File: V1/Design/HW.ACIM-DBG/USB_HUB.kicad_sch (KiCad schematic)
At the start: 45 parts, among them J1 USB C, U1 LDO 3.3V, U2 USB HUB 2.0 4-CH, Y1 24MHz

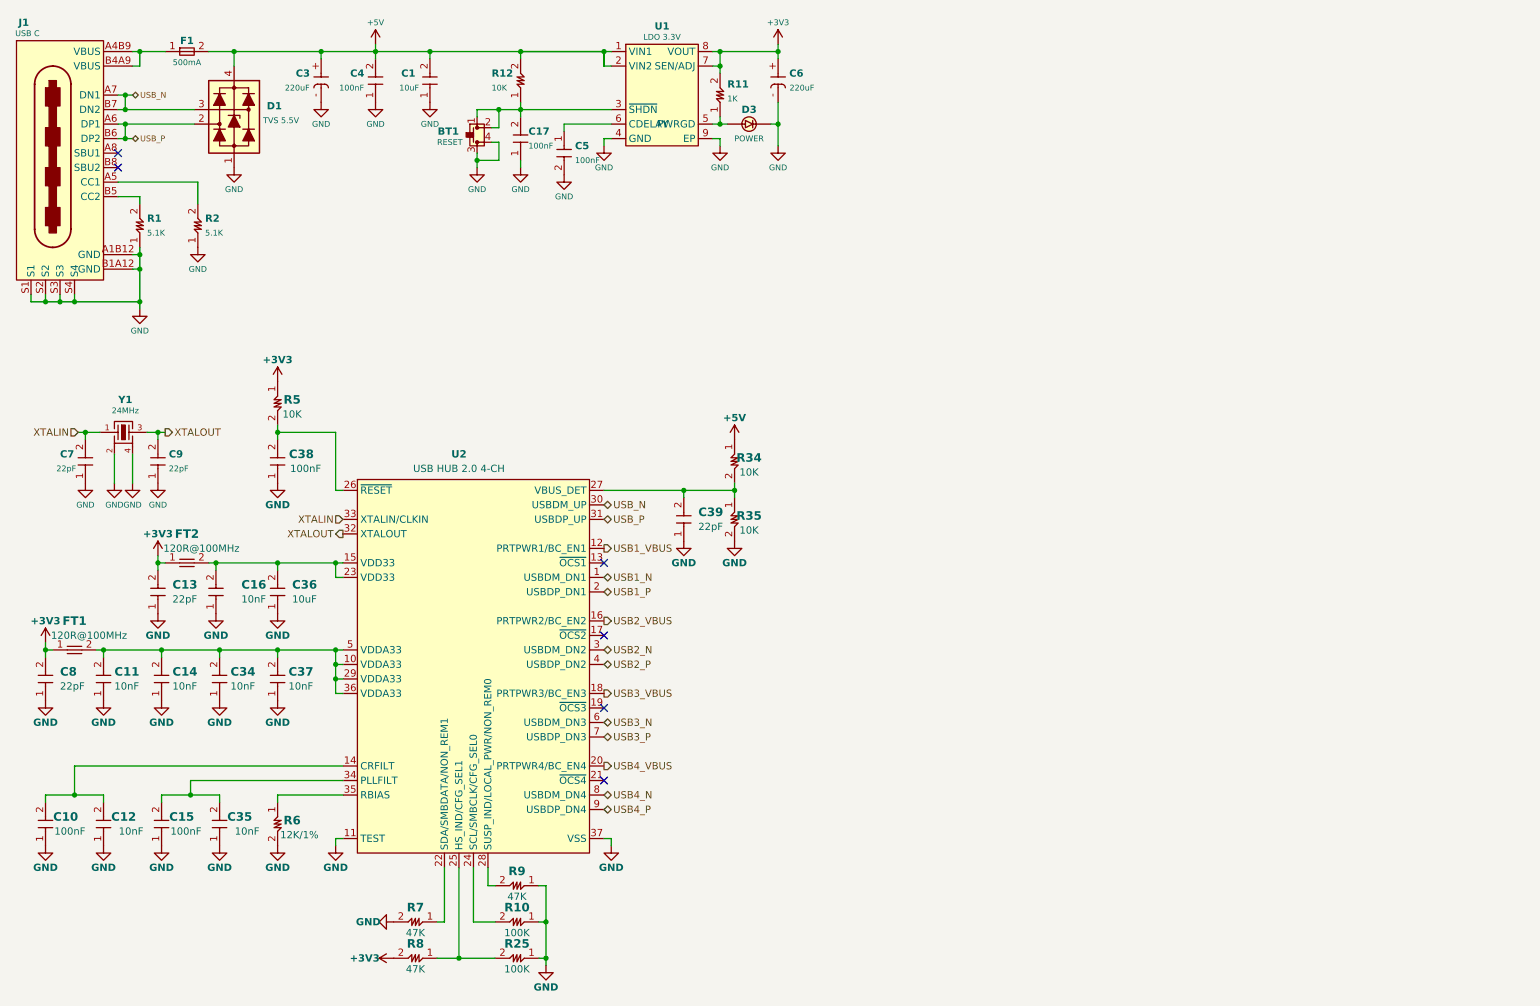
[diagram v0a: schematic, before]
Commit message: V1 layout update 6
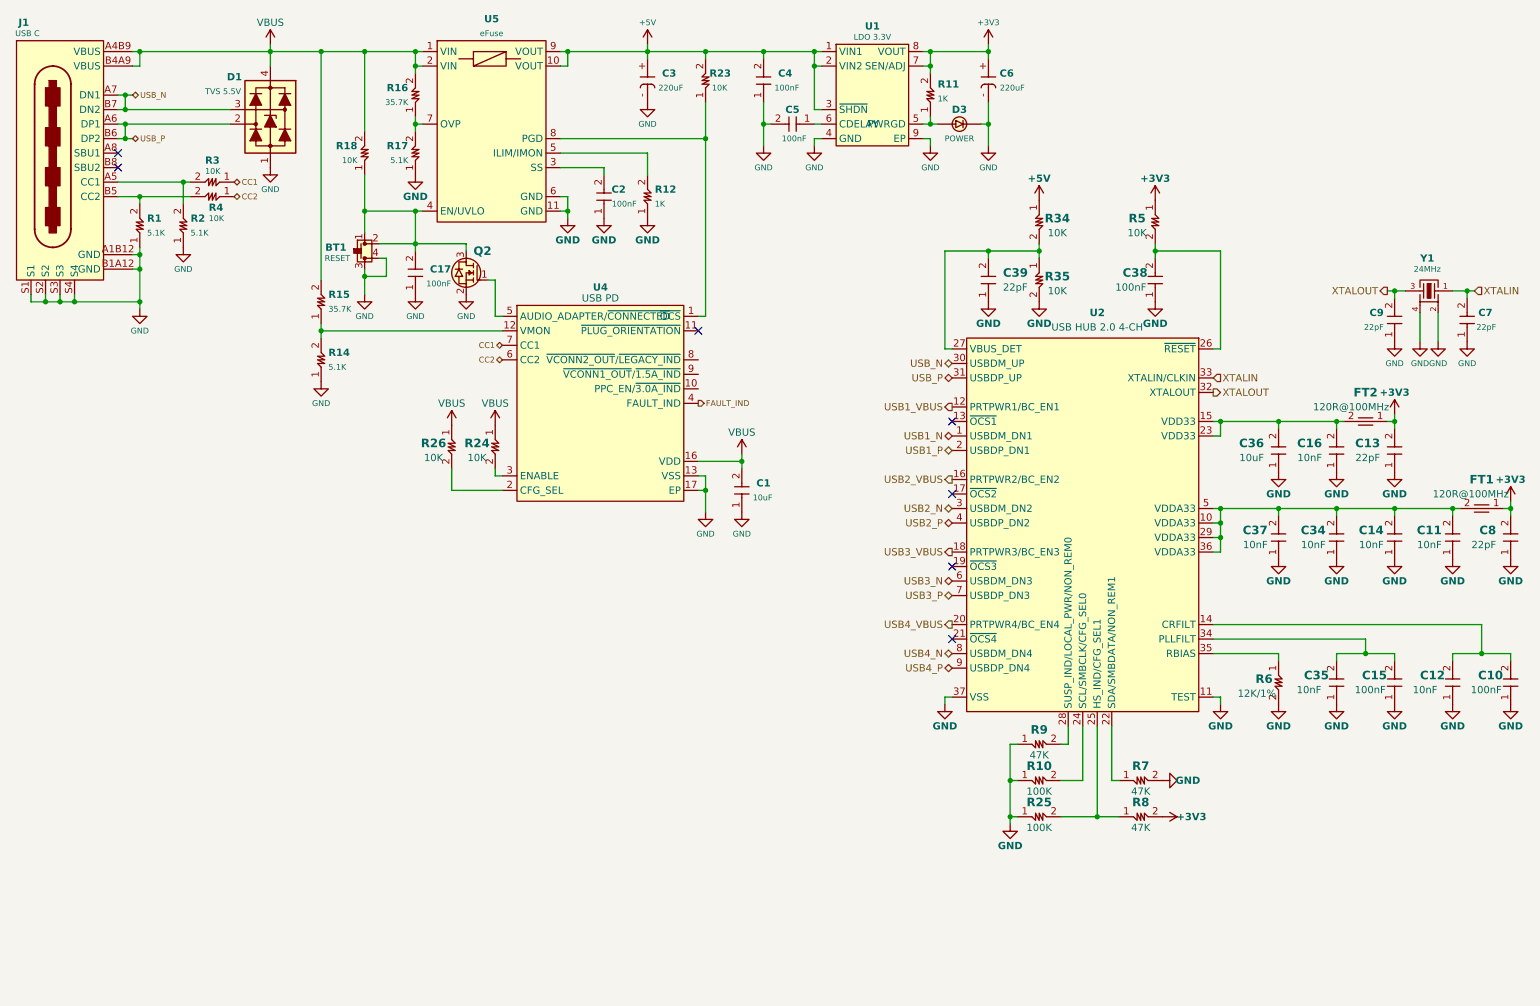
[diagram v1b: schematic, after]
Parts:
- removed F1: 500mA, SAMPI:FUSE0805, symbol Liem:FUSE
- added C2: 100nF, SAMPI:CAP0603, symbol SAMPI:CERCAP
- added Q2: MFET N, SAMPI:SOT23, symbol SAMPI:FET_N-CH
- added R14, R17: 5.1K, SAMPI:RES0603, symbol SAMPI:RES
- added R15, R16: 35.7K, SAMPI:RES0603, symbol SAMPI:RES
- added R18, R23, R24, R26, R3, R4: 10K, SAMPI:RES0603, symbol SAMPI:RES
- added U4: USB PD, SAMPI:QFN16, symbol Liem:UTC2000
- added U5: eFuse, SAMPI:DFN10-EP-3x3, symbol SAMPI:eFUSE
- D3: footprint SAMPI:LED3MM -> SAMPI:LED0603
- R12: value 10K -> 1K; MNP RC0603FR-0710KL -> RC0603FR-071KL
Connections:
- net +5V: now also U1.3 (~{SHDN}), R23.2, U5.10 (VOUT), U5.9 (VOUT); no longer C1.2, D1.4 (VCC), R12.2
- net GND: now also R12.1, C2.1, Q2.2 (S), R14.1, R17.1, U4.13 (VSS), U4.17 (EP), U5.11 (GND), U5.6 (GND)
- net at J1.A5 (CC1), R2.2: now also R3.2
- net at J1.B5 (CC2), R1.2: now also R4.2
- net at BT1.1, BT1.2, C17.2: now also Q2.3 (D), R18.1, U5.4 (EN/UVLO); no longer R12.1, U1.3 (~{SHDN})
- net VBUS: now reaches J1.A4B9 (VBUS), J1.B4A9 (VBUS)
- net VBUS: now also C1.2, D1.4 (VCC), R15.2, R16.2, R18.2, R24.1, R26.1, U4.16 (VDD), U5.1 (VIN), U5.2 (VIN)
- new net: R26.2, U4.2 (CFG_SEL)
- new net: R14.2, R15.1, U4.12 (VMON)
- new net: C2.2, U5.3 (SS)
- new net: R16.1, R17.2, U5.7 (OVP)
- new net: Q2.1 (G), U4.5 (AUDIO_ADAPTER/~{CONNECTED})
- new net: R23.1, U4.1 (~{OCS}), U5.8 (PGD)
- new net: R24.2, U4.3 (ENABLE)
- new net: R12.2, U5.5 (ILIM/IMON)
- new net CC1: R3.1, U4.7 (CC1)
- new net CC2: R4.1, U4.6 (CC2)
- new net FAULT_IND: U4.4 (FAULT_IND)
- no-connect marks 6 -> 7
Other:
- moved on the sheet: BT1, C1, C10, C11, C12, C13, C14, C15, C16, C17, C3, C34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
